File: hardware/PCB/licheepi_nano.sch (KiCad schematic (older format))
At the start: 4 parts

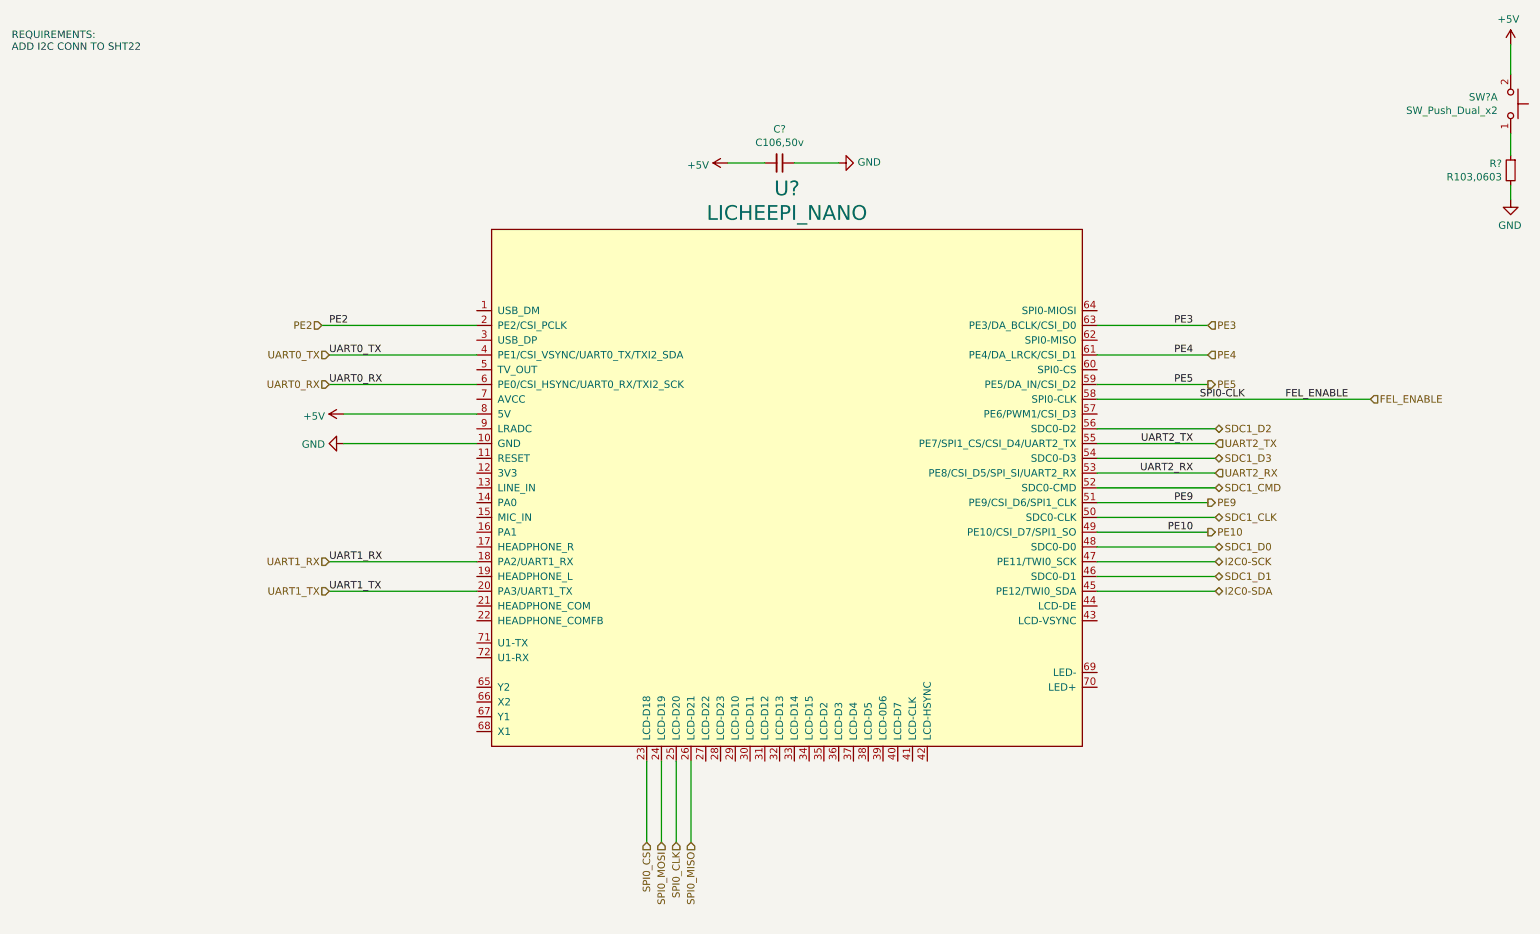
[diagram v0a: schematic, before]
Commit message: update for io_bank,
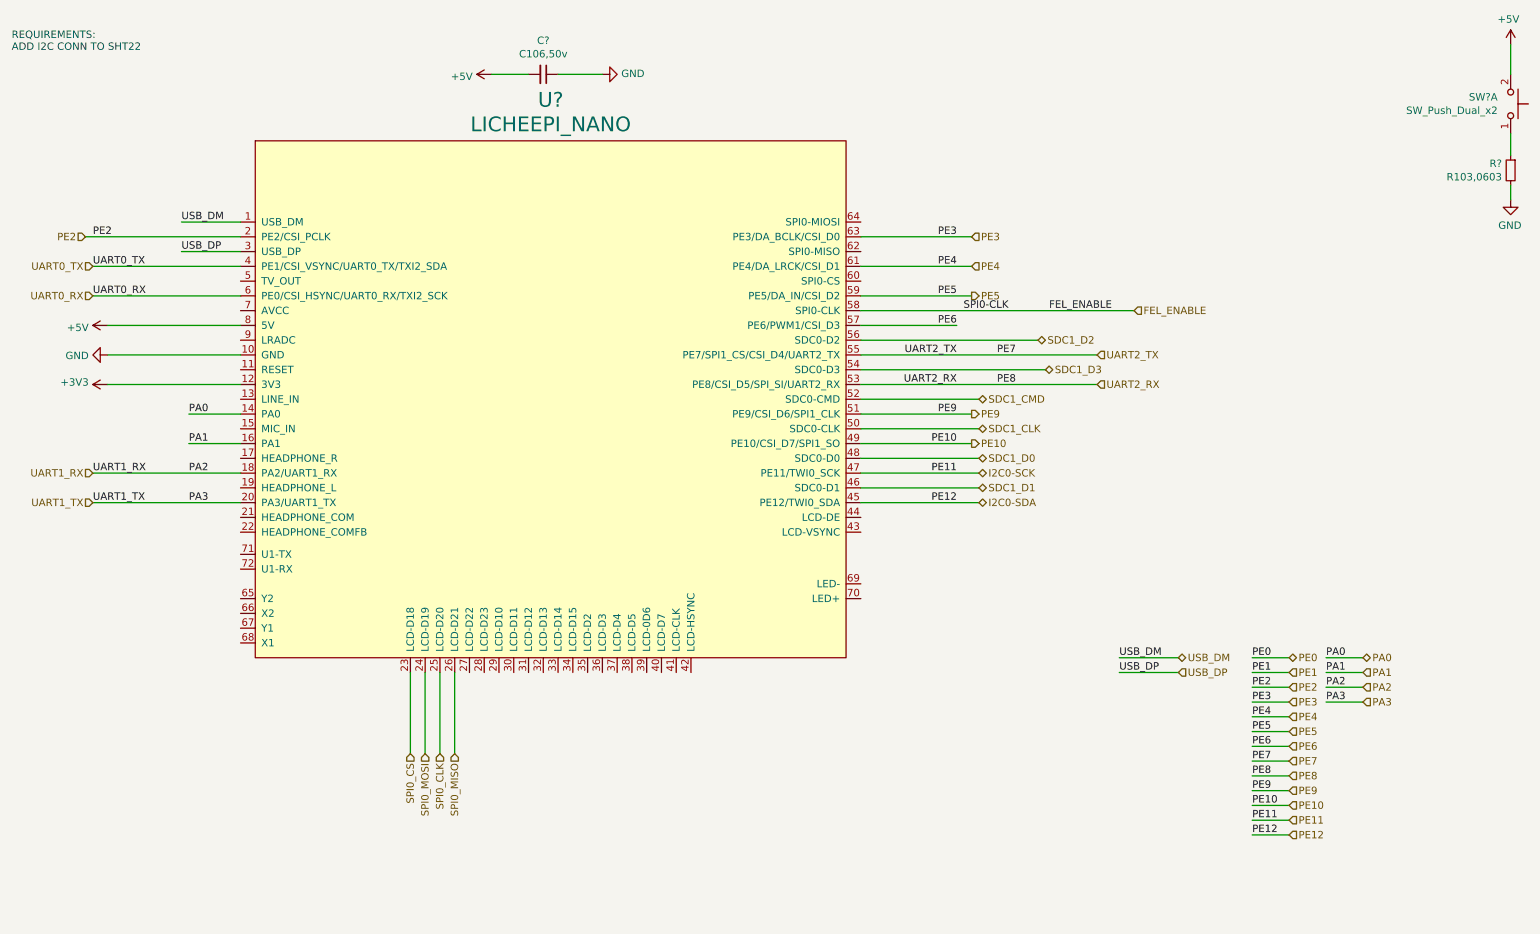
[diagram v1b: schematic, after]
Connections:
- net USB_DM: now reaches U?.1 (USB_DM)
- net +3V3: now reaches U?.12 (3V3)
- net PA0: now reaches U?.14 (PA0)
- net PA1: now reaches U?.16 (PA1)
- net USB_DP: now reaches U?.3 (USB_DP)
- net PE6: now reaches U?.57 (PE6/PWM1/CSI_D3)
- net UART1_RX renamed PA2
- net UART1_TX renamed PA3
- net UART2_RX renamed PE8
- net UART2_TX renamed PE7
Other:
- moved on the sheet: C?, U?
